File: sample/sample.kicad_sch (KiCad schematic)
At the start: 93 parts, among them M1 PMOS4pin, M10 NMOS3pin_1, M11 PMOS3pin_1, M12 NMOS3pin_2, M13 PMOS3pin_2, M14 NMOS4pin, M15 PMOS4pin, M2 PMOS4pin, M3 PMOS4pin, M4 NMOS4pin, M5 NMOS4pin, M6 NMOS4pin, M7 NMOS4pin, M8 NMOS4pin, M9 NMOS3pin_1, Q1 NPN, Q2 PNP, SW1 SW_CMOS, SW2 SW_SPDT, SW3 SW_SPST_OFF, SW4 SW_SPST_ON, U1 V_{DD}, U10 D_FF_R, U11 or31, U12 D_FF_R, U13 D_FF_R, U14 not, U15 nor21, U16 nor21, U17 GND_Drafting, U18 GND_Drafting, U19 GND_Drafting, U2 V_{DD}, U20 GND_Drafting, U21 OP_AMP, U24 RS_FF, U25 OP_AMP, U26 nand21, U27 nor21, U28 RS_FF, U29 JK_FF, U3 V_{DD}, U30 MUX21, U31 OP_AMP, U32 nand31, U33 nor31, U35 Differential_AMP, U36 and21, U37 or21, U38 D_FF, U39 T_FF, U4 V_{DD}, U40 MUX31, U41 and31, U42 or31, U43 Differential_AMP, U44 D_FF_R, U45 not, U46 xnor21, U47 MUX41, U48 VDD_Drafting, U49 buf, U5 V_{DD}, U50 xnor31, U51 GND_Drafting, U52 D_FF_R_S, U53 xor21, U54 xor31, U6 nand21, U7 delay, U8 D_FF_R, U9 D_FF_R

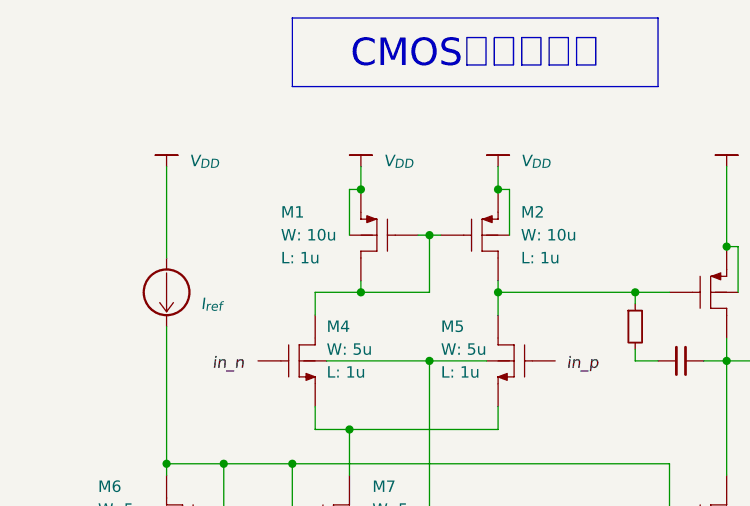
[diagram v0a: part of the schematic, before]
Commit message: サンプルの修正
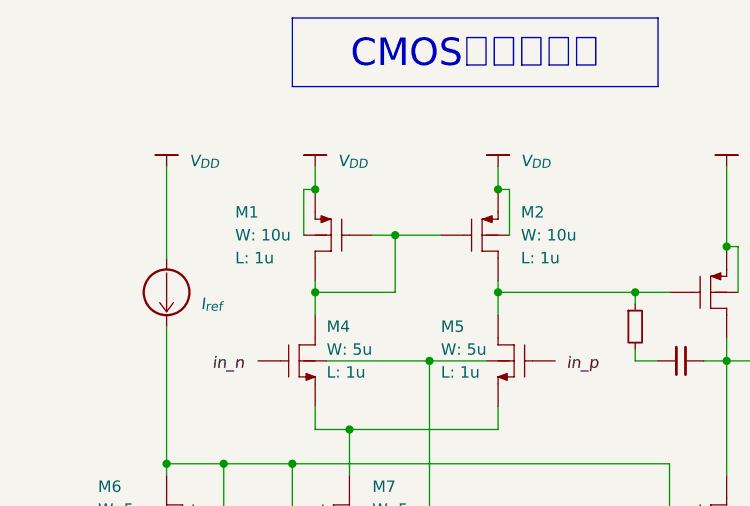
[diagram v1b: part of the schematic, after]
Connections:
- net at U24.1 (~Q): now also M9.1 (S)
- net at U25.1 (out): no longer U24.1 (~Q)
- net at U21.1 (out): no longer U24.1 (~Q)
- net at M9.1 (S): no longer U24.1 (~Q)
- net at U7.1 (Y): now also U10.1 (R), U9.1 (~Q); no longer U11.1 (Y)
- net at U9.1 (~Q): now also U10.1 (R), U13.1 (R)
- new net: U24.1 (~Q), U25.1 (out)
- new net: U21.1 (out), U24.1 (~Q)
- new net: U6.1 (Y), U8.1 (~Q)
- new net: U15.1 (Y), U8.1 (~Q)
- new net: U11.1 (Y), U7.1 (Y)
- new net: U12.1 (R), U14.1 (Y), U8.1 (~Q)
- new net: U16.1 (Y), U9.1 (~Q)
- new net: U10.1 (R), U13.1 (R), U9.1 (~Q)
- new net: U12.1 (R), U8.1 (~Q)
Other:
- moved on the sheet: M1
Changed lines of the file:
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@@
   (junction (at 220.98 71.12) (diameter 0) (color 0 0 0 0)
   )
-  (junction (at 54.61 39.37) (diameter 0) (color 0 0 0 0)
+  (junction (at 49.53 39.37) (diameter 0) (color 0 0 0 0)
+  )
+  (junction (at 58.42 44.45) (diameter 0) (color 0 0 0 0)
   )
   (junction (at 228.6 76.2) (diameter 0) (color 0 0 0 0)
@@
   (junction (at 33.02 69.85) (diameter 0) (color 0 0 0 0)
   )
-  (junction (at 62.23 44.45) (diameter 0) (color 0 0 0 0)
-  )
   (junction (at 85.09 50.8) (diameter 0) (color 0 0 0 0)
   )
@@
   (junction (at 95.25 58.42) (diameter 0) (color 0 0 0 0)
   )
-  (junction (at 54.61 50.8) (diameter 0) (color 0 0 0 0)
-  )
   (junction (at 52.07 125.095) (diameter 0) (color 0 0 0 0)
   )
@@
   (junction (at 172.72 53.34) (diameter 0) (color 0 0 0 0)
   )
+  (junction (at 49.53 50.8) (diameter 0) (color 0 0 0 0)
+  )
   (junction (at 62.23 58.42) (diameter 0) (color 0 0 0 0)
   )
@@
     (stroke (width 0) (type default))
   )
-  (wire (pts (xy 62.23 50.8) (xy 62.23 44.45))
+  (wire (pts (xy 58.42 50.8) (xy 58.42 44.45))
     (stroke (width 0) (type default))
   )
@@
   )
   (wire (pts (xy 53.34 83.82) (xy 53.34 81.28))
-    (stroke (width 0) (type default))
-  )
-  (wire (pts (xy 49.53 50.8) (xy 54.61 50.8))
     (stroke (width 0) (type default))
   )
@@
     (stroke (width 0) (type default))
   )
+  (wire (pts (xy 49.53 50.8) (xy 58.42 50.8))
+    (stroke (width 0) (type default))
+  )
   (wire (pts (xy 195.58 49.53) (xy 198.12 49.53))
     (stroke (width 0) (type default))
@@
     (stroke (width 0) (type default))
   )
-  (wire (pts (xy 53.34 39.37) (xy 54.61 39.37))
+  (wire (pts (xy 48.26 39.37) (xy 49.53 39.37))
     (stroke (width 0) (type default))
   )
@@
     (stroke (width 0) (type default))
   )
-  (wire (pts (xy 62.23 44.45) (xy 60.96 44.45))
-    (stroke (width 0) (type default))
-  )
-  (wire (pts (xy 54.61 36.83) (xy 54.61 39.37))
+  (wire (pts (xy 49.53 36.83) (xy 49.53 39.37))
     (stroke (width 0) (type default))
   )
@@
     (stroke (width 0) (type default))
   )
+  (wire (pts (xy 58.42 44.45) (xy 63.5 44.45))
+    (stroke (width 0) (type default))
+  )
   (wire (pts (xy 71.12 106.045) (xy 71.12 115.57))
     (stroke (width 0) (type default))
@@
     (stroke (width 0) (type default))
   )
-  (wire (pts (xy 53.34 44.45) (xy 53.34 39.37))
+  (wire (pts (xy 48.26 44.45) (xy 48.26 39.37))
     (stroke (width 0) (type default))
   )
@@
     (stroke (width 0) (type default))
   )
-  (wire (pts (xy 54.61 50.8) (xy 62.23 50.8))
-    (stroke (width 0) (type default))
-  )
-  (wire (pts (xy 62.23 44.45) (xy 63.5 44.45))
-    (stroke (width 0) (type default))
-  )
   (wire (pts (xy 39.37 69.85) (xy 46.99 69.85))
     (stroke (width 0) (type default))
@@
     (stroke (width 0) (type default))
   )
-  (wire (pts (xy 54.61 49.53) (xy 54.61 50.8))
+  (wire (pts (xy 49.53 49.53) (xy 49.53 50.8))
     (stroke (width 0) (type default))
   )
@@
   )
   (wire (pts (xy 49.53 63.5) (xy 49.53 66.04))
+    (stroke (width 0) (type default))
+  )
+  (wire (pts (xy 58.42 44.45) (xy 55.88 44.45))
     (stroke (width 0) (type default))
   )
@@
     )
   )
-  (symbol (lib_id "Drafting_Symbols:VDD_Drafting") (at 54.61 36.83 0) (unit 1)
-    (in_bom yes) (on_board yes) (dnp no) (fields_autoplaced)
-    (property "Reference" "U2" (at 54.61 34.29 0)
-      (effects (font (size 1.27 1.27)) hide)
-    )
-    (property "Value" "V_{DD}" (at 57.15 36.195 0)
+  (symbol (lib_id "Drafting_Symbols:VDD_Drafting") (at 49.53 36.83 0) (unit 1)
+    (in_bom yes) (on_board yes) (dnp no) (fields_autoplaced)
+    (property "Reference" "U2" (at 49.53 34.29 0)
+      (effects (font (size 1.27 1.27)) hide)
+    )
+    (property "Value" "V_{DD}" (at 52.07 36.195 0)
       (effects (font (size 1.27 1.27) italic) (justify left))
     )
-    (property "Footprint" "" (at 54.61 34.29 0)
-      (effects (font (size 1.27 1.27)) hide)
-    )
-    (property "Datasheet" "" (at 54.61 34.29 0)
+    (property "Footprint" "" (at 49.53 34.29 0)
+      (effects (font (size 1.27 1.27)) hide)
+    )
+    (property "Datasheet" "" (at 49.53 34.29 0)
       (effects (font (size 1.27 1.27)) hide)
     )
@@
     )
   )
-  (symbol (lib_name "PMOS4pin_1") (lib_id "Drafting_Symbols:PMOS4pin") (at 54.61 44.45 0) (mirror y) (unit 1)
+  (symbol (lib_name "PMOS4pin_1") (lib_id "Drafting_Symbols:PMOS4pin") (at 49.53 44.45 0) (mirror y) (unit 1)
     (in_bom yes) (on_board yes) (dnp no)
-    (property "Reference" "M1" (at 45.72 41.91 0)
+    (property "Reference" "M1" (at 40.64 41.91 0)
       (effects (font (size 1.27 1.27)) (justify right))
     )
-    (property "Value" "PMOS4pin" (at 55.88 38.1 0)
-      (effects (font (size 1.27 1.27)) hide)
-    )
-    (property "Footprint" "" (at 55.88 38.1 0)
-      (effects (font (size 1.27 1.27)) hide)
-    )
-    (property "Datasheet" "" (at 55.88 38.1 0)
-      (effects (font (size 1.27 1.27)) hide)
-    )
-    (property "W" "10u" (at 45.72 44.45 0) (show_name)
+    (property "Value" "PMOS4pin" (at 50.8 38.1 0)
+      (effects (font (size 1.27 1.27)) hide)
+    )
+    (property "Footprint" "" (at 50.8 38.1 0)
+      (effects (font (size 1.27 1.27)) hide)
+    )
+    (property "Datasheet" "" (at 50.8 38.1 0)
+      (effects (font (size 1.27 1.27)) hide)
+    )
+    (property "W" "10u" (at 40.64 44.45 0) (show_name)
       (effects (font (size 1.27 1.27)) (justify right))
     )
-    (property "L" "1u" (at 45.72 46.99 0) (show_name)
+    (property "L" "1u" (at 40.64 46.99 0) (show_name)
       (effects (font (size 1.27 1.27)) (justify right))
     )
-    (property "M" "" (at 54.61 44.45 0)
+    (property "M" "" (at 49.53 44.45 0)
       (effects (font (size 1.27 1.27)) (justify left))
     )
